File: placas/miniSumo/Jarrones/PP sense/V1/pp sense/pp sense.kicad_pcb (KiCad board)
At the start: 2 copper layers, 100.1 x 39.4 mm, 41 parts, among them J1 Conn_01x07_Pin, Q1 BC547, Q2 BC547, Q3 BC547, Q4 BC547, U1 LM339

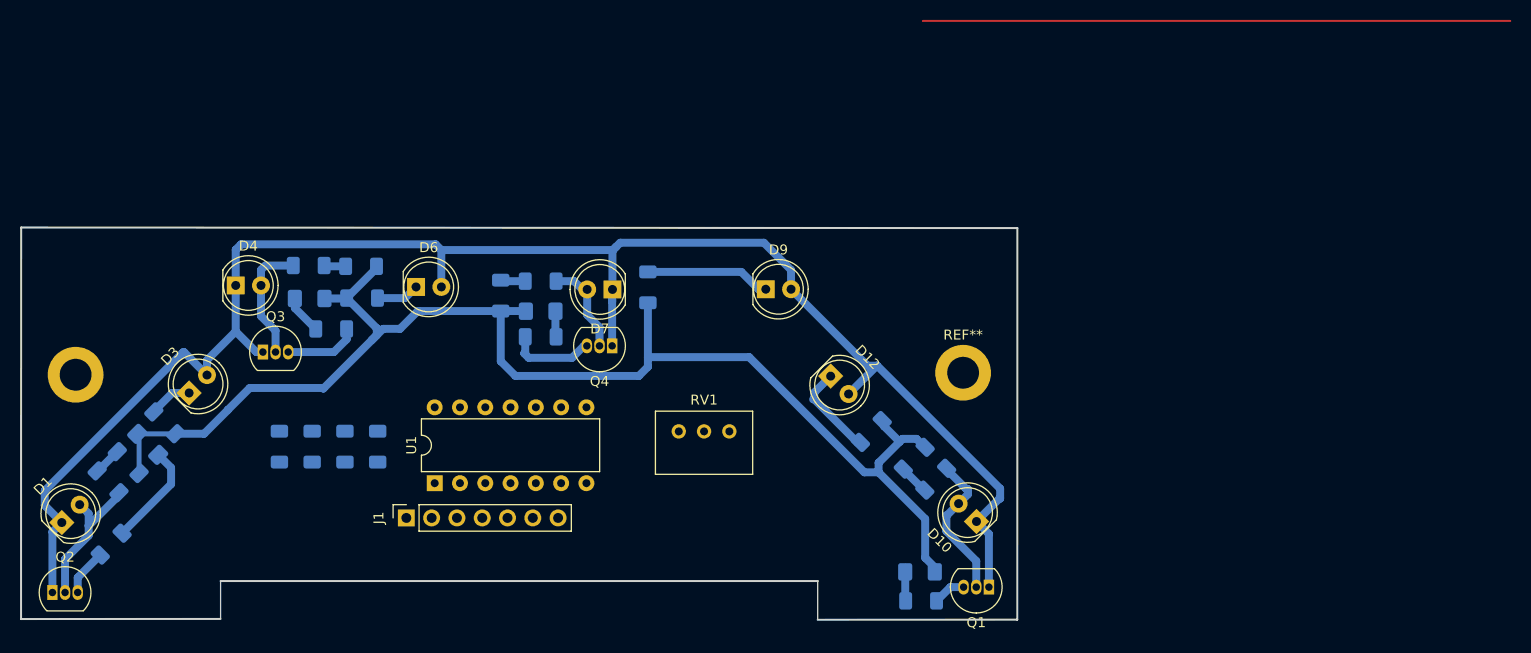
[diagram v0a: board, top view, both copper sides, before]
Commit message: gfgf
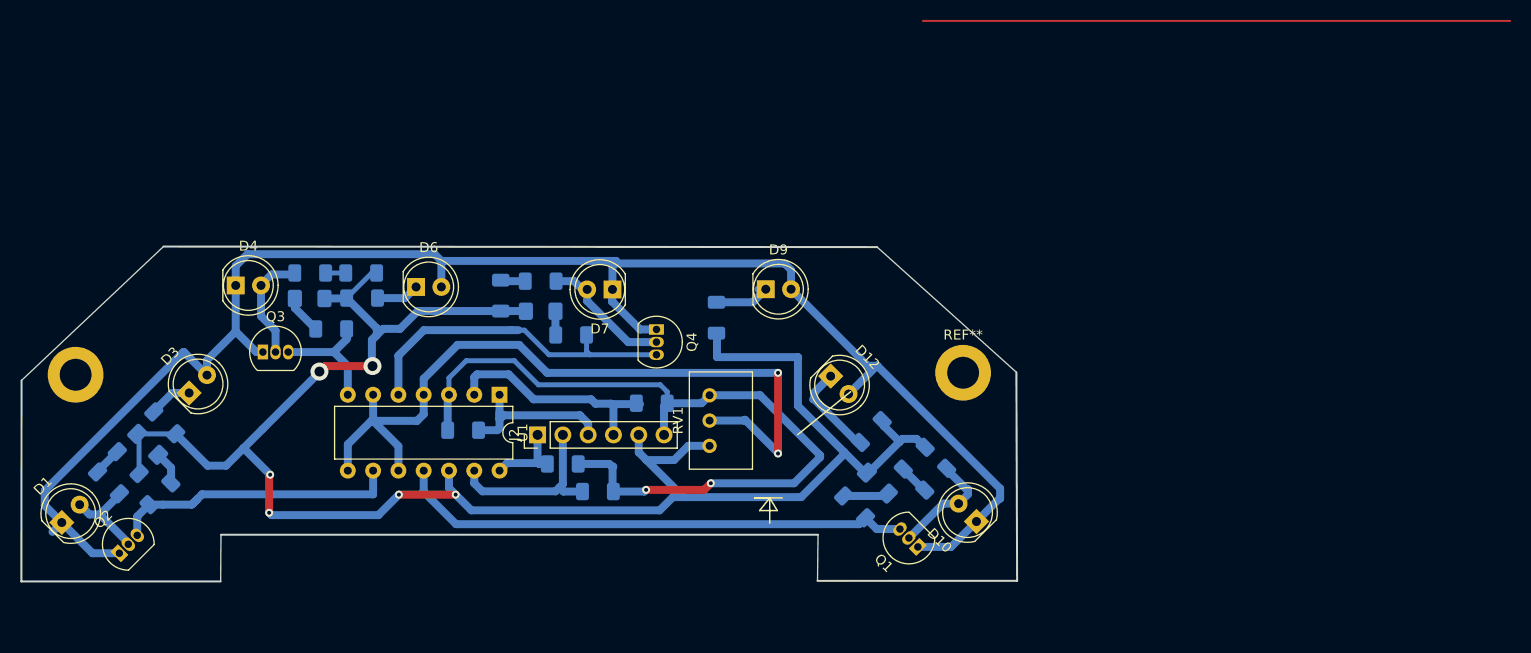
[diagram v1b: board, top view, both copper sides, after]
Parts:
- removed J1: Conn_01x07_Pin, Connector_PinSocket_2.54mm:PinSocket_1x07_P2.54mm_Vertical
- removed the R3 at (29.3, 100.2)
- added J2: Conn_01x06_Pin, Connector_PinHeader_2.54mm:PinHeader_1x06_P2.54mm_Vertical, F.Cu at (72.4, 95.5)
- added R20: 1k, Resistor_SMD:R_1206_3216Metric_Pad1.30x1.75mm_HandSolder, B.Cu at (29.3, 100.3)
- moved R17 29.1 mm to (78.5, 101.2), turned to 0 degrees
- moved R3 28.5 mm to (75.0, 98.4), turned to 0 degrees
- moved R19 27.9 mm to (83.9, 92.3), turned to 0 degrees
- moved R18 12.0 mm to (65.0, 95.0), turned to 180 degrees
- moved R13 11.6 mm to (104.3, 102.8), turned to 135 degrees
- moved U1 11.0 mm to (68.6, 91.5), turned to -90 degrees
- moved D11 9.89 mm to (106.6, 100.4), turned to -45 degrees
- moved Q1 8.20 mm to (110.6, 106.8), turned to 135 degrees
- moved Q2 7.80 mm to (30.4, 107.4), turned to 45 degrees
- moved R16 7.53 mm to (90.4, 83.8)
- moved R1 7.04 mm to (34.5, 101.4)
- moved Q4 4.75 mm to (84.4, 84.9), turned to -90 degrees
- moved RV1 4.14 mm to (89.7, 91.5), turned to 90 degrees
- moved R9 3.07 mm to (75.8, 85.5), turned to 180 degrees
- moved R7 0.76 mm to (49.6, 79.3)
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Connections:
- Q1 pad 3: /D4 -> /D3
- Q2 pad 3: /D3 -> /D4
- R1 pad 1: /D3 -> /D4
- R13 pad 1: /D4 -> /D3
- R17 pad 2: Net-(J1-Pin_2) -> +5V
- R18 pad 2: Net-(J1-Pin_3) -> +5V
- R19 pad 2: Net-(J1-Pin_4) -> +5V
- R2 pad 2: unconnected-(R2-Pad2) -> Net-(R2-Pad2)
- R3 pad 2: Net-(J1-Pin_1) -> +5V
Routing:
- net +5V: track 0.00 -> 80.6 mm, vias 0 -> 2
- net Net-(U1A--): track 0.00 -> 78.6 mm, vias 0 -> 2
- net GND: track 137.5 -> 187.3 mm, vias 0 -> 6
- net /D3: track 4.70 -> 52.1 mm
- net /D1: track 8.67 -> 34.8 mm
- net /D4: track 3.35 -> 29.4 mm
- net Net-(J2-Pin_4): track 0.00 -> 23.0 mm
- net Net-(J2-Pin_2): track 0.00 -> 18.2 mm
- net Net-(J2-Pin_3): track 0.00 -> 16.8 mm
- net Net-(J2-Pin_1): track 0.00 -> 8.09 mm
- net Net-(D2-A): track 10.9 -> 3.49 mm
- net Net-(D9-K): track 12.6 -> 6.21 mm
- net Net-(D1-A): track 14.8 -> 9.60 mm
- net /D2: track 7.55 -> 12.4 mm
- net Net-(D10-A): track 15.4 -> 11.7 mm
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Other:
- board size 100.1 x 39.4 mm -> 100 x 33.6 mm
